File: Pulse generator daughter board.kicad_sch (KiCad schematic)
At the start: 61 parts, among them J1 Vin1, J10 Vin2_GND, J11 DVM1_ADC, J12 GND, J13 DVM2_ADC, J14 GND, J15 PWM1 input, J16 PWM2 input, J17 CH1 output, J18 GND, J19 CH2 output, J2 Vin1_GND, J20 GND, J3 3V3, J4 DVM1, J5 GND, J6 3V3, J7 DVM2, J8 GND, J9 Vin2, U1 TC4427, U2 TC4427

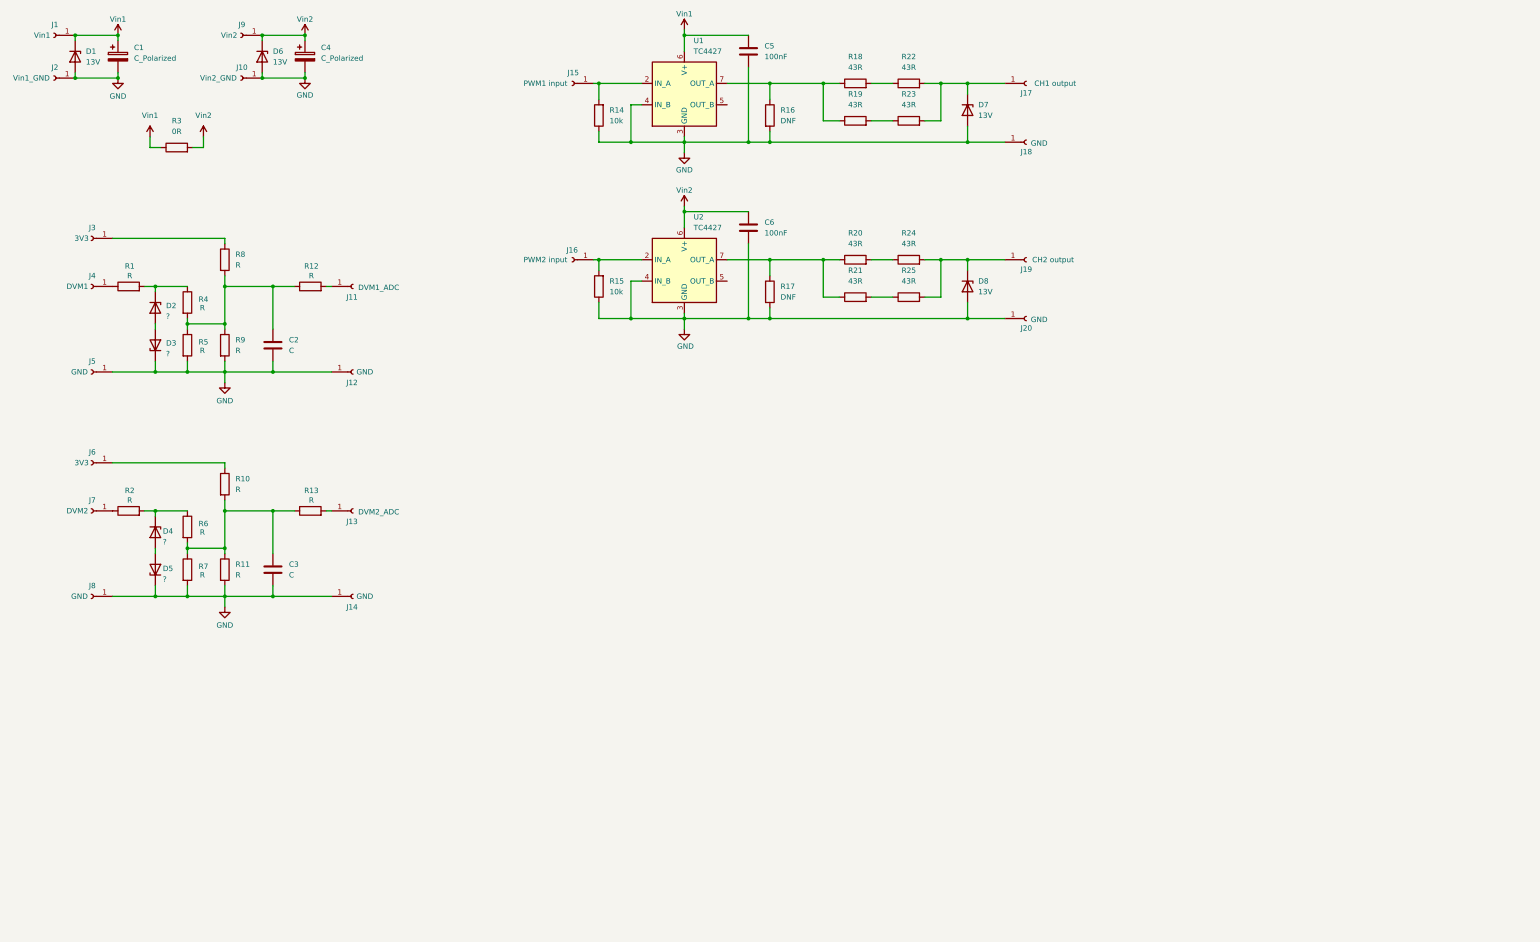
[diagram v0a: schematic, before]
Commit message: Progress 2 on schematic and PCB
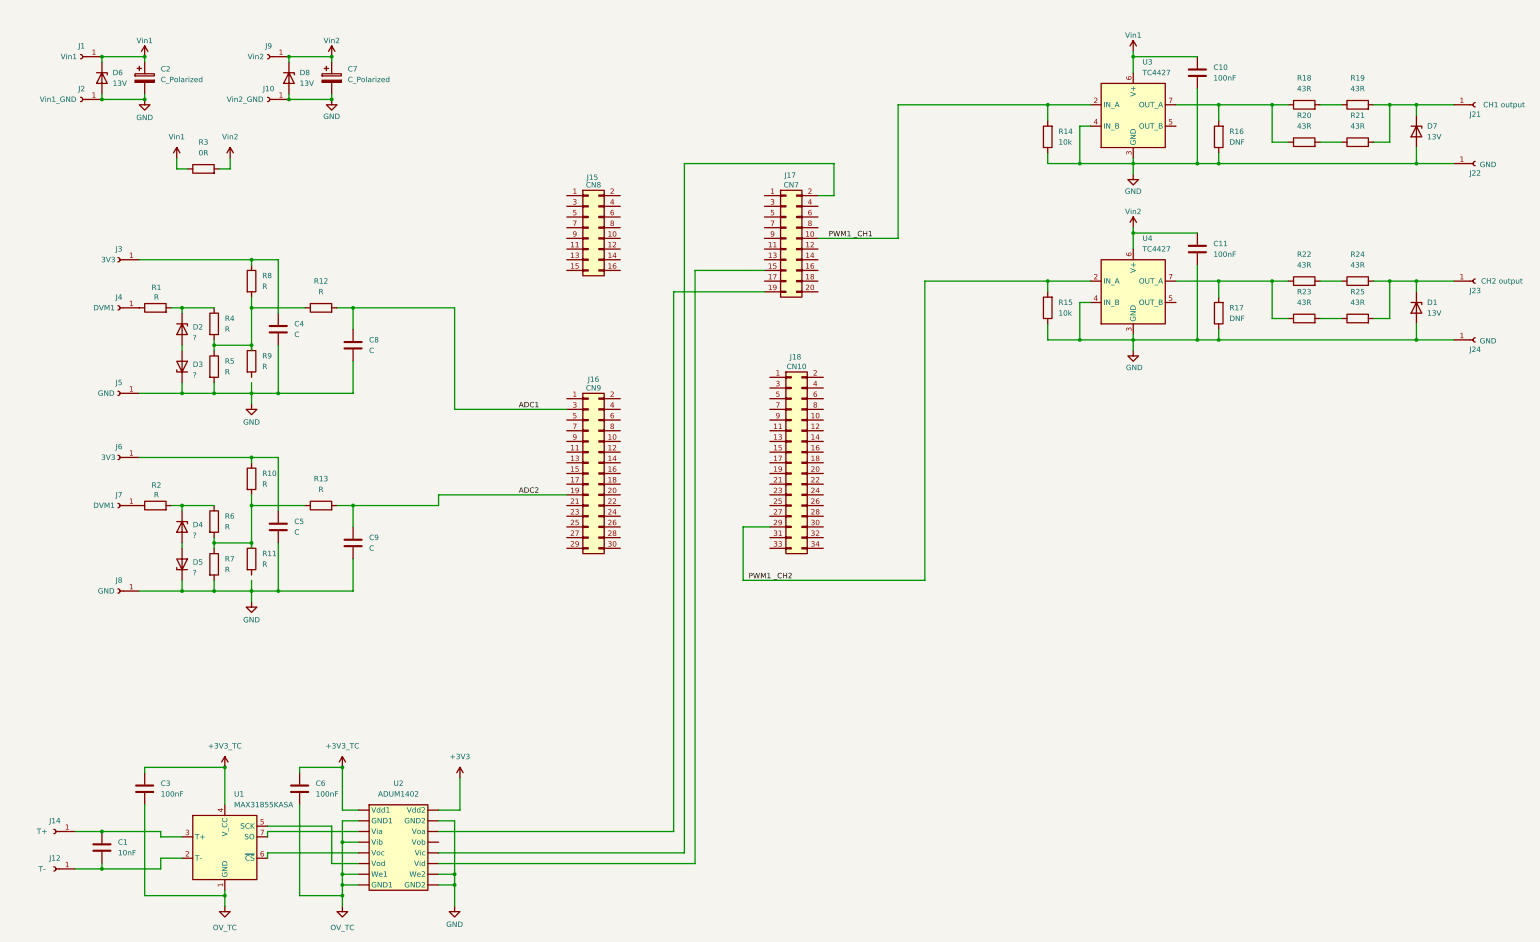
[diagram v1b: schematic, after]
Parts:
- removed J11: DVM1_ADC, symbol Connector:Conn_01x01_Socket
- removed J13: DVM2_ADC, symbol Connector:Conn_01x01_Socket
- removed J15: PWM1 input, symbol Connector:Conn_01x01_Socket
- removed J16: PWM2 input, symbol Connector:Conn_01x01_Socket
- added C1: 10nF, symbol Device:C
- added C4, C5, C9: C, symbol Device:C
- added C6: 100nF, symbol Device:C
- added J15: CN8, Connector_PinHeader_2.54mm:PinHeader_2x08_P2.54mm_Vertical, symbol Connector_Generic:Conn_02x08_Odd_Even
- added J16: CN9, Connector_PinHeader_2.54mm:PinHeader_2x15_P2.54mm_Vertical, symbol Connector_Generic:Conn_02x15_Odd_Even
- added J17: CN7, Connector_PinHeader_2.54mm:PinHeader_2x10_P2.54mm_Vertical, symbol Connector_Generic:Conn_02x10_Odd_Even
- added J18: CN10, Connector_PinHeader_2.54mm:PinHeader_2x17_P2.54mm_Vertical, symbol Connector_Generic:Conn_02x17_Odd_Even
- added U1: MAX31855KASA, Package_SO:SOIC-8_3.9x4.9mm_P1.27mm, symbol Sensor_Temperature:MAX31855KASA
- added U2: ADUM1402, Package_SO:SOIC-16W_7.5x10.3mm_P1.27mm, symbol Rafal_Library:ADUM1402
- C3: value C -> 100nF
- D1, D6, D7, D8: footprint (none) -> Diode_SMD:D_SMA_Handsoldering
- J12: value GND -> T-
- J14: value GND -> T+
- J7: value DVM2 -> DVM1
- R10, R11, R12, R13, R14, R15, R16, R17, R3, R4, R5, R6, R7, R8, R9: footprint (none) -> Resistor_SMD:R_0805_2012Metric_Pad1.20x1.40mm_HandSolder
- R18, R19, R20, R21, R22, R23, R24, R25: footprint (none) -> Resistor_SMD:R_2512_6332Metric_Pad1.40x3.35mm_HandSolder
- renumbered C5 to C10, C6 to C11, C1 to C2, C4 to C7, C2 to C8, J17 to J21, J18 to J22, J19 to J23, J20 to J24, U1 to U3, U2 to U4
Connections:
- net GND: now also R16.1, R17.1, C4.2, C5.2, C9.2, U2. (We2); no longer C3.2, J12.1 (Pin_1), J14.1 (Pin_1), R11.2, R16.2, R17.2, R9.2
- net Vin1: now also D6.1 (K); no longer D1.1 (K)
- net Vin2: now also D8.1 (K); no longer D6.1 (K)
- net at J6.1 (Pin_1), R10.1: now also C5.1
- net PWM1 _CH1: now reaches R14.2, U3.2 (IN_A)
- net PWM1 _CH1: now also J17.10 (Pin_10)
- net ADC2: now reaches R13.2
- net ADC2: now also C9.1, J16.19 (Pin_19)
- net at R10.2, R11.1, R13.1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: no longer C3.1
- net at D7.1 (K), J21.1 (Pin_1): now also R19.2, R21.2; no longer R22.2, R23.2
- net at R25.1: now also R23.2; no longer R21.2
- net at J23.1 (Pin_1), R24.2, R25.2: now also D1.1 (K); no longer D8.1 (K)
- net PWM1 _CH2: now reaches R15.2, U4.2 (IN_A)
- net PWM1 _CH2: now also J18.29 (Pin_29)
- net at R18.1, U3.7 (OUT_A): now also R16.2, R20.1; no longer R16.1, R19.1
- net at J3.1 (Pin_1), R8.1: now also C4.1
- net at R12.1, R4.2, R5.1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: no longer C8.1
- net at R18.2: now also R19.1; no longer R22.1
- net at R24.1: now also R22.2; no longer R20.2
- net at R23.1: now also R17.2, R22.1, U4.7 (OUT_A); no longer R19.2
- net ADC1: now reaches R12.2
- net ADC1: now also C8.1, J16.3 (Pin_3)
- new net: J17.15 (Pin_15), U2. (We2)
- new net: J17.19 (Pin_19), U2. (We2)
- new net: J17.2 (Pin_2), U2. (We2)
- new net: C1.1, J14.1 (Pin_1), U1.3 (T+)
- new net: C1.2, J12.1 (Pin_1), U1.2 (T-)
- new net: R20.2, R21.1
- new net: U1.5 (SCK), U2. (We2)
- new net: U1.6 (~{CS}), U2. (We2)
- new net: U1.7 (SO), U2. (We2)
- new net +3V3: U2. (We2)
- new net +3V3_TC: C3.1, C6.1, U1.4 (V_CC), U2. (We2)
- new net OV_TC: C3.2, C6.2, U1.1 (GND), U2. (We2)
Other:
- moved on the sheet: C10, C11, C2, C7, C8, D2, D3, D7, J1, J10, J2, J21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
